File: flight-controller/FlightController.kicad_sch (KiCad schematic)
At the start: 13 parts, among them J1 USB_C_Receptacle_USB2.0_14P, U1 ESP32-S3-WROOM-1, U2 TPS629210

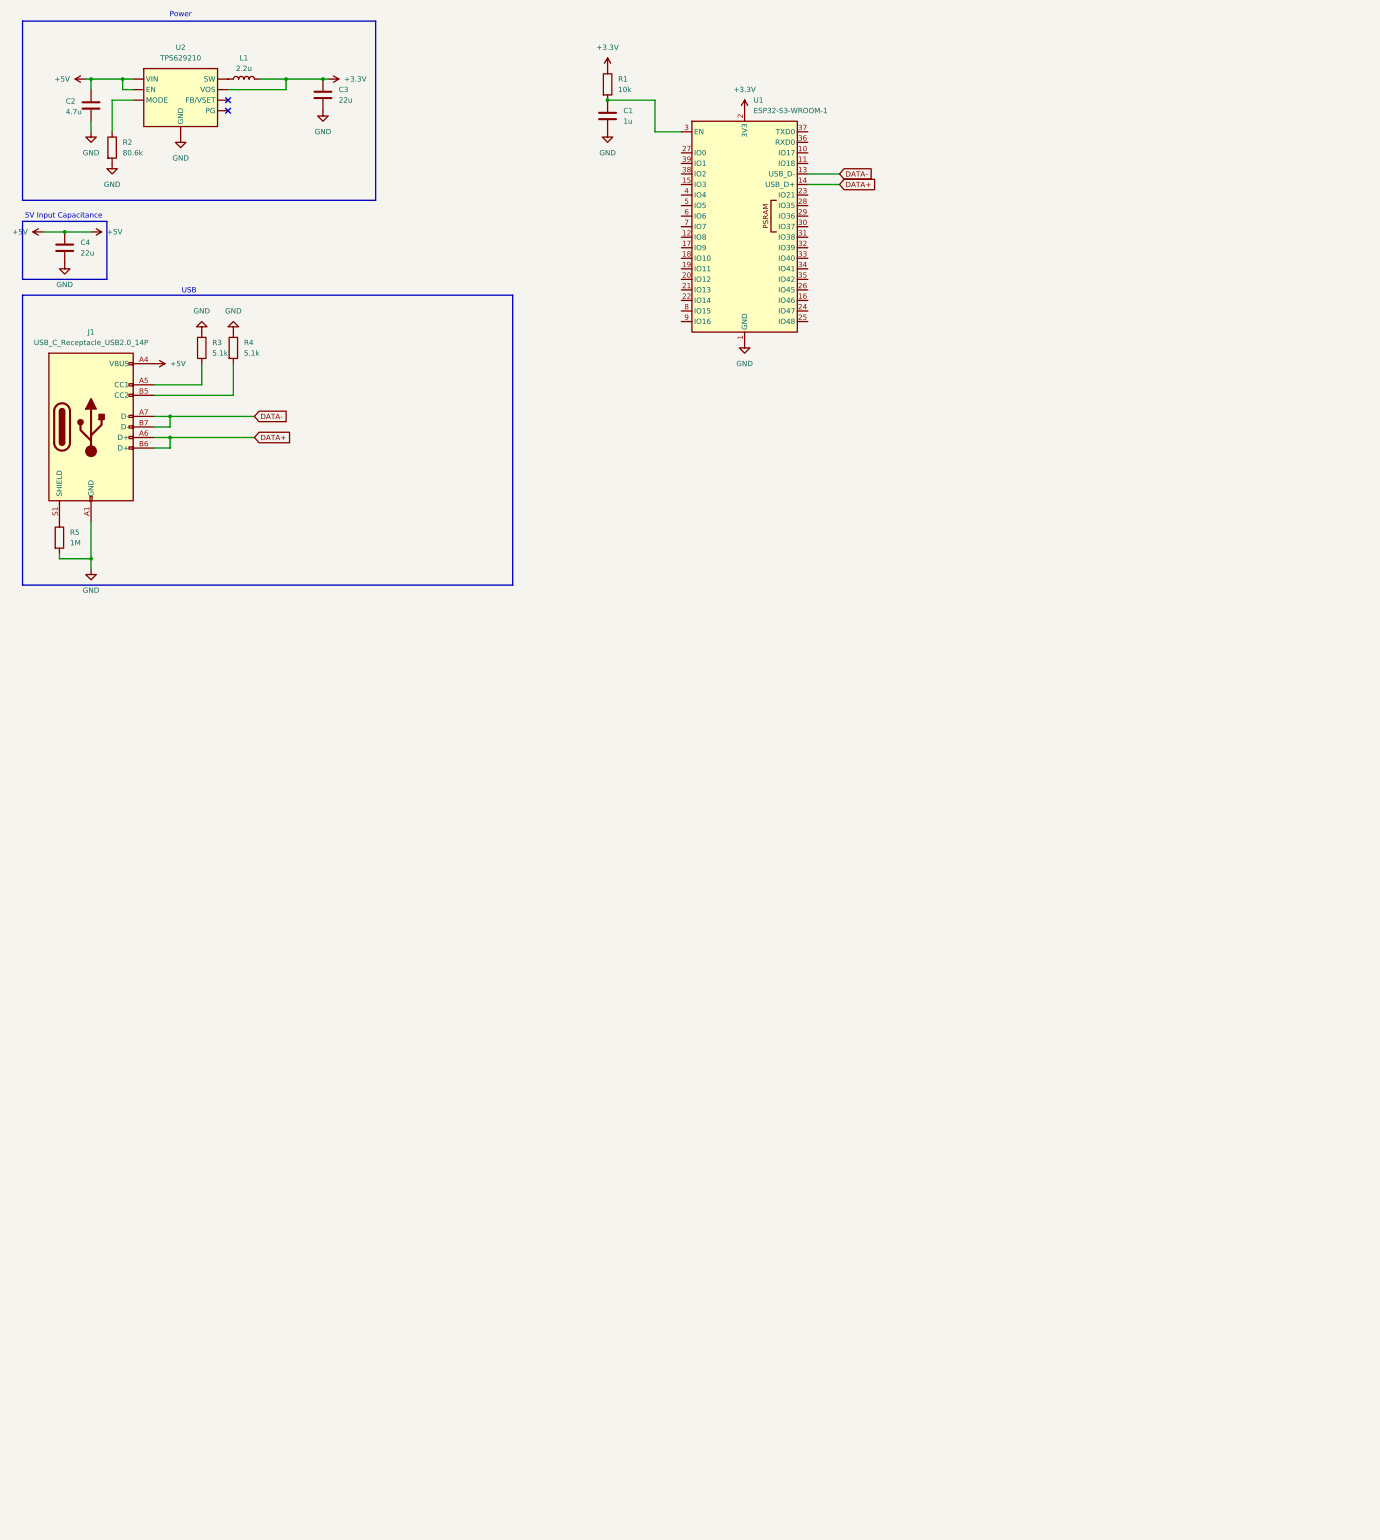
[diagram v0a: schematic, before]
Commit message: Add a bunch of sensors
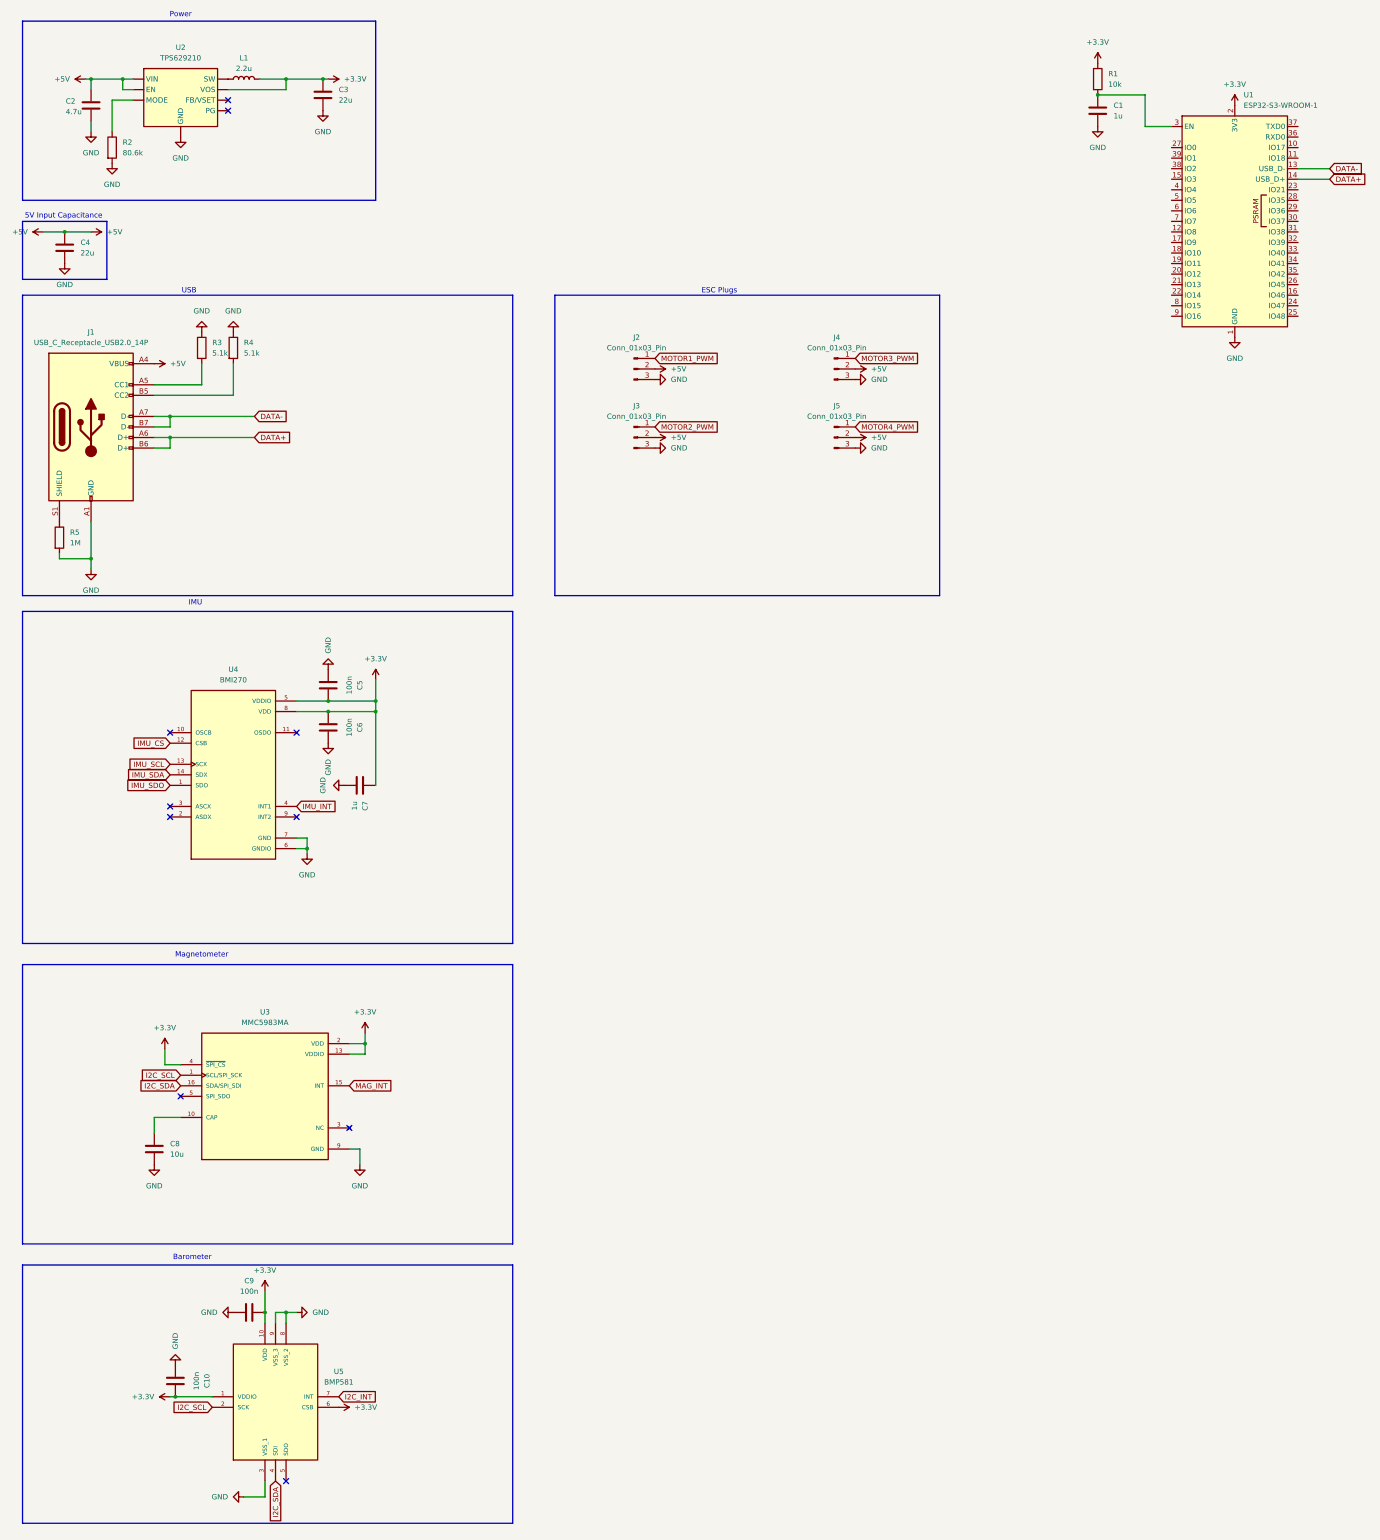
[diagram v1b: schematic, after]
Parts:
- added C10, C5, C6, C9: 100n, symbol Device:C
- added C7: 1u, symbol Device:C
- added C8: 10u, symbol Device:C
- added J2, J3, J4, J5: Conn_01x03_Pin, symbol Connector:Conn_01x03_Pin
- added U3: MMC5983MA, MMC5983MA:PQFN50P300X300X100-16N, symbol MMC5983MA:MMC5983MA
- added U4: BMI270, BMI270:XDCR_BMI270, symbol BMI270:BMI270
- added U5: BMP581, BMP581:BMP581, symbol BMP581:BMP581
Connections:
- net +3.3V: now also C10.2, C5.2, C6.1, C7.2, C9.2, U3.13 (VDDIO), U3.2 (VDD), U3.4 (~{SPI_CS}), U4.5 (VDDIO), U4.8 (VDD), U5.1 (VDDIO), U5.10 (VDD), U5.6 (CSB)
- net +5V: now also J2.2 (Pin_2), J3.2 (Pin_2), J4.2 (Pin_2), J5.2 (Pin_2)
- net GND: now also C10.1, C5.1, C6.2, C7.1, C8.2, C9.1, J2.3 (Pin_3), J3.3 (Pin_3), J4.3 (Pin_3), J5.3 (Pin_3), U3.11 (GND), U3.9 (GND), U4.6 (GNDIO), U4.7 (GND), U5.3 (VSS_1), U5.8 (VSS_2), U5.9 (VSS_3)
- new net: C8.1, U3.10 (CAP)
- new net: U3.12 (NC), U3.14 (NC), U3.3 (NC), U3.6 (NC), U3.7 (NC), U3.8 (NC)
- new net I2C_INT: U5.7 (INT)
- new net I2C_SCL: U3.1 (SCL/SPI_SCK), U5.2 (SCK)
- new net I2C_SDA: U3.16 (SDA/SPI_SDI), U5.4 (SDI)
- new net IMU_CS: U4.12 (CSB)
- new net IMU_INT: U4.4 (INT1)
- new net IMU_SCL: U4.13 (SCX)
- new net IMU_SDA: U4.14 (SDX)
- new net IMU_SDO: U4.1 (SDO)
- new net MAG_INT: U3.15 (INT)
- new net MOTOR1_PWM: J2.1 (Pin_1)
- new net MOTOR2_PWM: J3.1 (Pin_1)
- new net MOTOR3_PWM: J4.1 (Pin_1)
- new net MOTOR4_PWM: J5.1 (Pin_1)
- no-connect marks 2 -> 10
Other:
- note added: "Barometer"
- note added: "ESC Plugs"
- note added: "IMU"
- note added: "Magnetometer"
- moved on the sheet: C1, R1, U1
